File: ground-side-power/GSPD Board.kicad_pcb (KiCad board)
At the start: 2 copper layers, 286.6 x 219.2 mm, 94 parts, among them J1 Battery Terminals, J10 Conn_01x03_Female, J12 Conn_01x04_Female, J13 DAQ Voltage Sensing, J14 DAQ Current Sensing, J15 To Router, J16 To RLCS, J17 To DAQ Laptop, J18 Conn_01x02_Female, J19 Conn_01x02_Female, J2 Battery Terminals, J20 To Ethernet, J21 To 5V M12, J22 To DAQ, J23 Extra M12, J24 Extra M12, J25 Extra M12, J26 Conn_01x02_Female, J27 Conn_01x02_Female, J3 Battery Terminals, J4 Battery Terminals, J5 874270842, J6 874270842, J7 ATX-24, J8 Conn_01x03_Female, J9 Conn_01x03_Female, K1 AZ2150-1A-12DEF, M1 Fan_PC_Chassis, M2 Fan_PC_Chassis, SW1 GRB234A2NABA1, U1 INA180, U2 INA180, U3 K7805-3AR3, U4 INA180, U5 INA180, U6 URB2424LD-20WR3

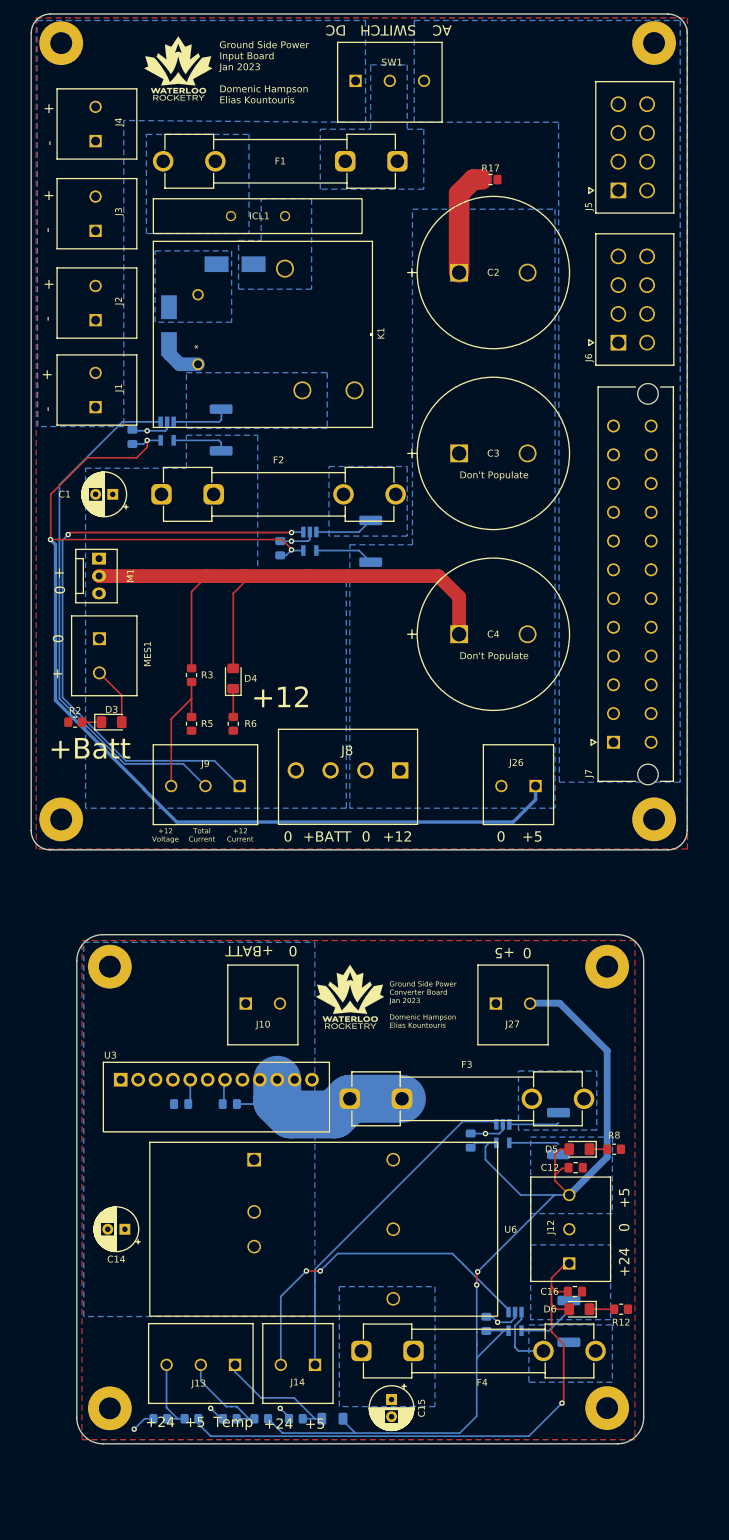
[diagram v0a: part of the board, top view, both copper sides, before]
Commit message: Added Gerbers
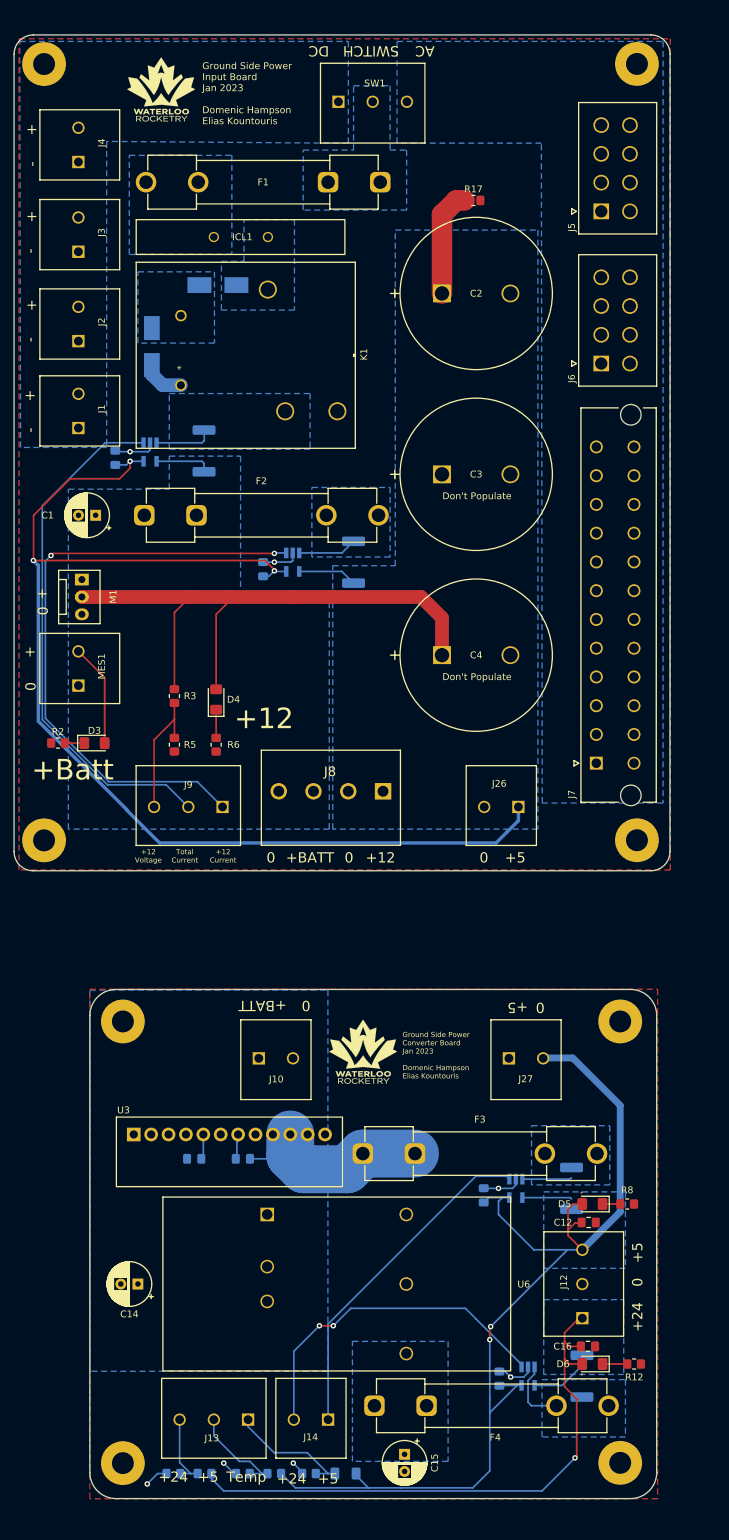
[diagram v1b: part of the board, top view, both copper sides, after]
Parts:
- removed the ? at (28.1, -113.9)
- removed the ? at (100.7, -49.5)
- removed the ? at (107.6, -131.3)
- removed the ? at (100.7, -113.9)
- removed the ? at (21.0, -131.2)
- removed the ? at (107.6, -244.6)
- removed the ? at (28.1, -49.4)
- removed the G*** at (38.1, -240.9)
- removed the G*** at (63.2, -105.3)
- added ?: , clipboard:6b5716c7-8553-4764-af17-05841c85de2e, F.Cu at (30.0, -105.9)
- added ?: , clipboard:6b5716c7-8553-4764-af17-05841c85de2e, F.Cu at (30.0, -41.4)
- added ?: , , F.Cu at (18.5, -128.2)
- added ?: , clipboard:6b5716c7-8553-4764-af17-05841c85de2e, F.Cu at (102.6, -105.9)
- added ?: , , F.Cu at (105.1, -241.6)
- added ?: , , F.Cu at (105.1, -128.2)
- added ?: , clipboard:6b5716c7-8553-4764-af17-05841c85de2e, F.Cu at (102.6, -41.5)
- added G***: LOGO, rlcs:rocketry_logo_small, F.Cu at (35.6, -237.9)
- added G***: LOGO, rlcs:rocketry_logo_small, F.Cu at (65.1, -97.3)
- MES1: footprint GSP:OSTTA020161 -> GSP:1935310
- moved C11 8.22 mm to (40.4, -81.7)
- moved C12 8.22 mm to (98.0, -72.4)
- moved C15 8.22 mm to (71.1, -38.5)
- moved C16 8.22 mm to (97.9, -54.3)
- moved C9 8.22 mm to (82.7, -76.3)
- moved D5 8.22 mm to (98.6, -75.1)
- moved F3 8.22 mm to (65.0, -82.4)
- moved J10 8.22 mm to (49.8, -96.3)
- moved J27 8.22 mm to (86.4, -96.3)
- moved R10 8.22 mm to (41.9, -35.7)
- moved R11 8.22 mm to (52.1, -35.7)
- moved R13 8.22 mm to (37.3, -35.7)
- moved R15 8.22 mm to (62.5, -35.7)
- moved R16 8.22 mm to (57.1, -35.7)
- moved R8 8.22 mm to (103.6, -75.1)
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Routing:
- net +BATT: track 16.8 -> 23.3 mm
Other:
- board size 286.6 x 219.2 mm -> 289.1 x 216.1 mm
